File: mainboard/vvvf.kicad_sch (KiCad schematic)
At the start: 101 parts, among them J1 Conn_01x16_Pin, J2 Screw_Terminal_01x01, J3 Screw_Terminal_01x01, J4 Screw_Terminal_01x01, J5 Screw_Terminal_01x01, J6 Screw_Terminal_01x02, J7 Screw_Terminal_01x01, J8 Screw_Terminal_01x01, J9 Screw_Terminal_01x02, Q1 Q_NIGBT_GCE, Q2 Q_NIGBT_GCE, SW1 SW_Push, U1 TLP152, U11 LM7805_TO220, U12 AMC1303M2510DWVR, U2 TLP152, U3 UCC21520ADW, U4 TLP152, U5 ACS758KCB-150B-PFF-T, U6 UCC21520ADW, U7 UCC21520ADW, U8 ACS758KCB-150B-PFF-T, U9 ACS758KCB-150B-PFF-T

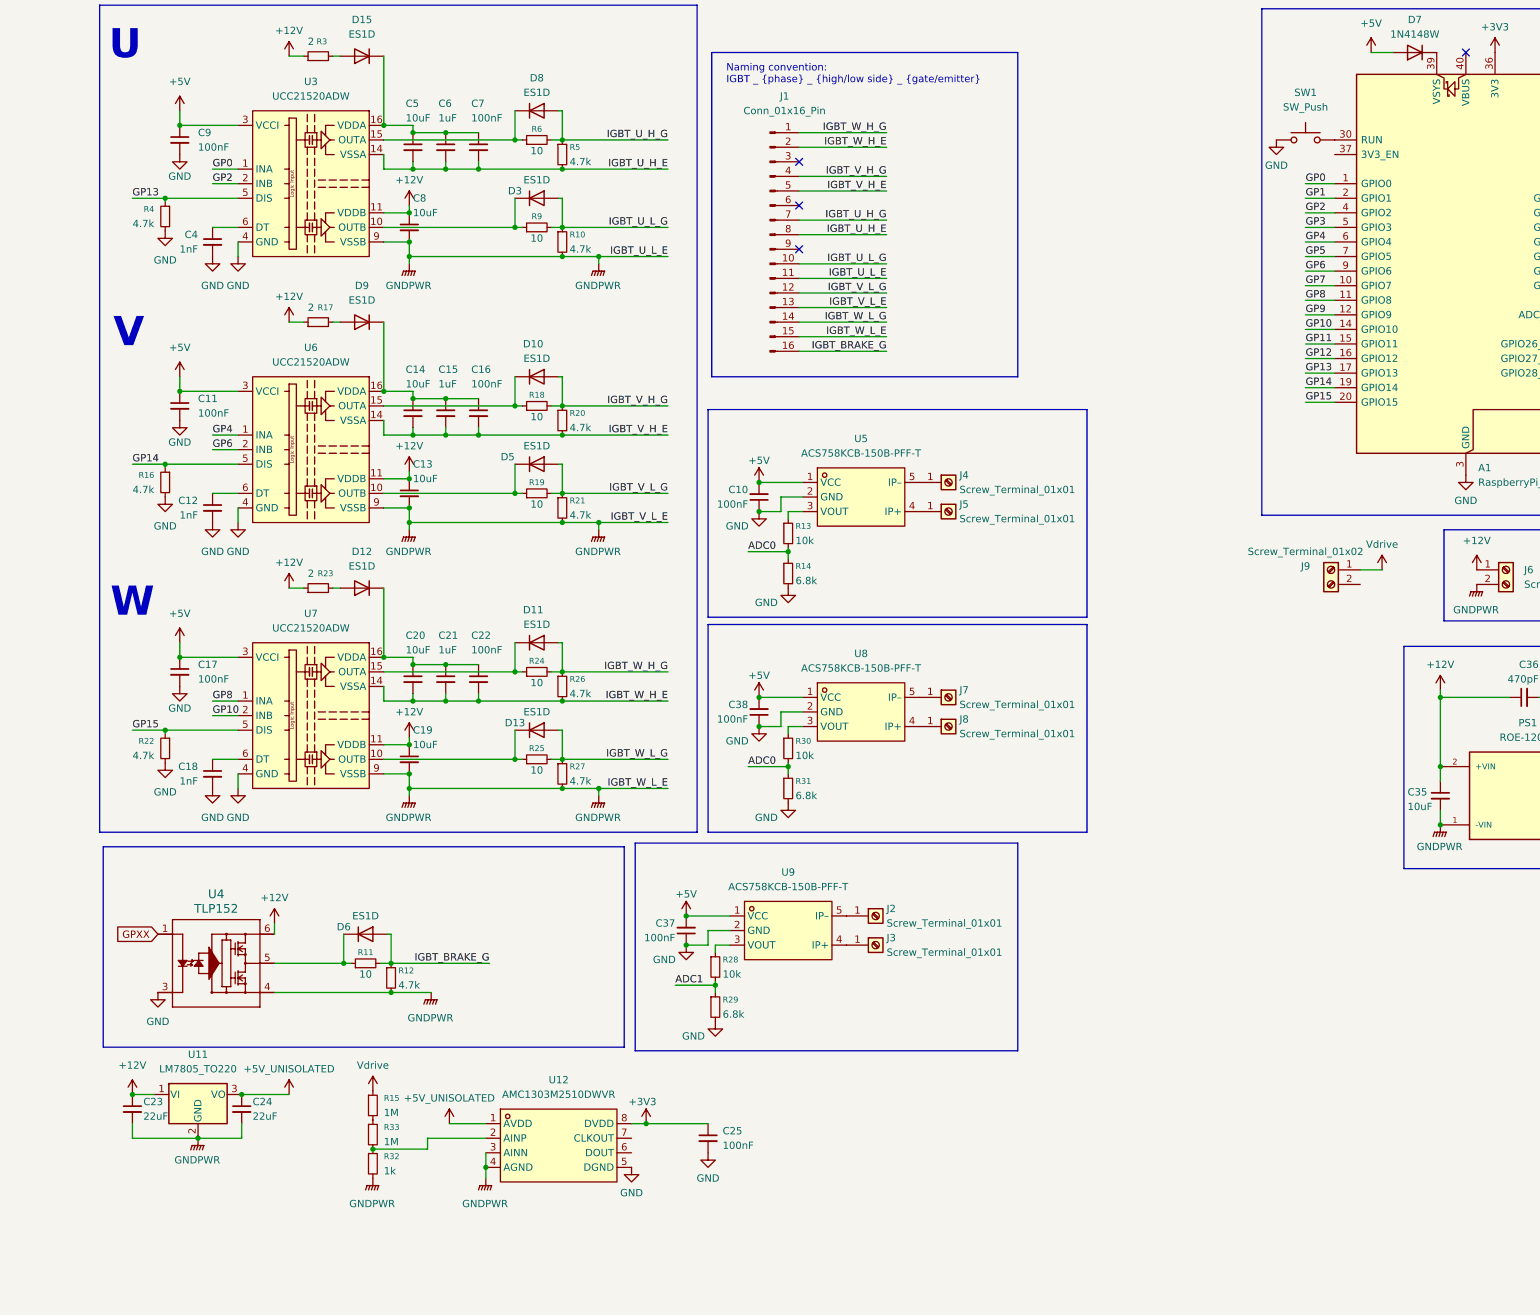
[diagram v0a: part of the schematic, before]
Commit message: current sense board
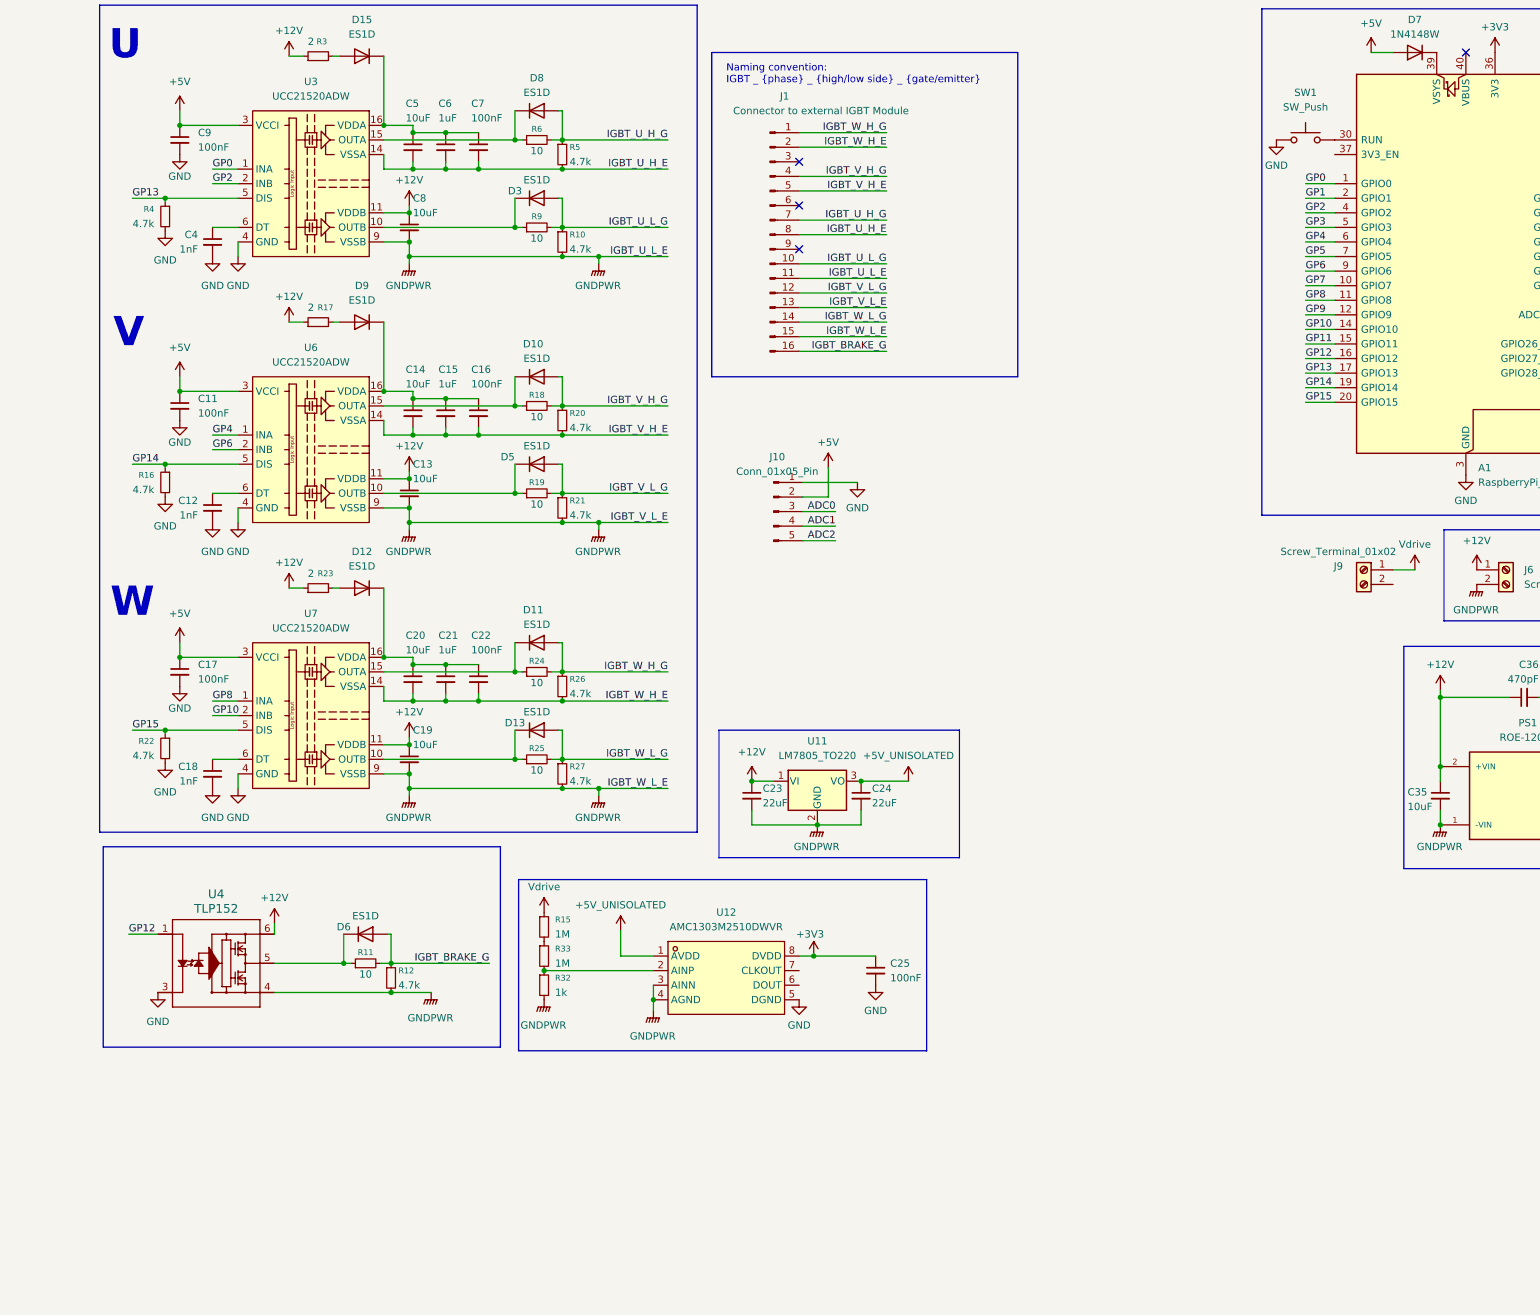
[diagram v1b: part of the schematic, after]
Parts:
- removed C10, C37, C38: 100nF, Capacitor_SMD:C_0603_1608Metric_Pad1.08x0.95mm_HandSolder, symbol Device:C_Small
- removed J2, J3, J4, J5, J7, J8: Screw_Terminal_01x01, easyeda2kicad:CONN-TH_T44001, symbol Connector:Screw_Terminal_01x01
- removed R13, R28, R30: 10k, Resistor_SMD:R_0603_1608Metric_Pad0.98x0.95mm_HandSolder, symbol Device:R_Small
- removed R14, R29, R31: 6.8k, Resistor_SMD:R_0603_1608Metric_Pad0.98x0.95mm_HandSolder, symbol Device:R_Small
- removed U5, U8, U9: ACS758KCB-150B-PFF-T, easyeda2kicad:SENSOR-TH_ACS758KCB-150B-PFF-T, symbol easyeda2kicad:ACS758KCB-150B-PFF-T_C6396159
- added J10: Conn_01x05_Pin, Connector_PinHeader_2.54mm:PinHeader_1x05_P2.54mm_Vertical, symbol Connector:Conn_01x05_Pin
- J1: value Conn_01x16_Pin -> Connector to external IGBT Module
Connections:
- net +5V: now also J10.2 (Pin_2)
- net ADC0: now also J10.3 (Pin_3)
- net ADC1: now also J10.4 (Pin_4)
- net ADC2: now also J10.5 (Pin_5)
- net GND: now also J10.1 (Pin_1)
- net GP12: now also U4.1
- net GPXX: no longer U4.1
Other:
- moved on the sheet: C23, C24, C25, J9, R15, R32, R33, U11, U12
